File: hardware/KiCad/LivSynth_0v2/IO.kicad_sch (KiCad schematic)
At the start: 95 parts, among them J1 PJ398SM, J13 Jumper, J14 Jumper, J2 PJ398SM, J20 IDC, J3 PJ398SM, J4 IDC, Q6 2N3904, Q7 2N3904, SW6 SW_Push, U10 PCA9685PW, U11 PCA9685PW, U13 74HC165, U14 74HC165, U3 LM386

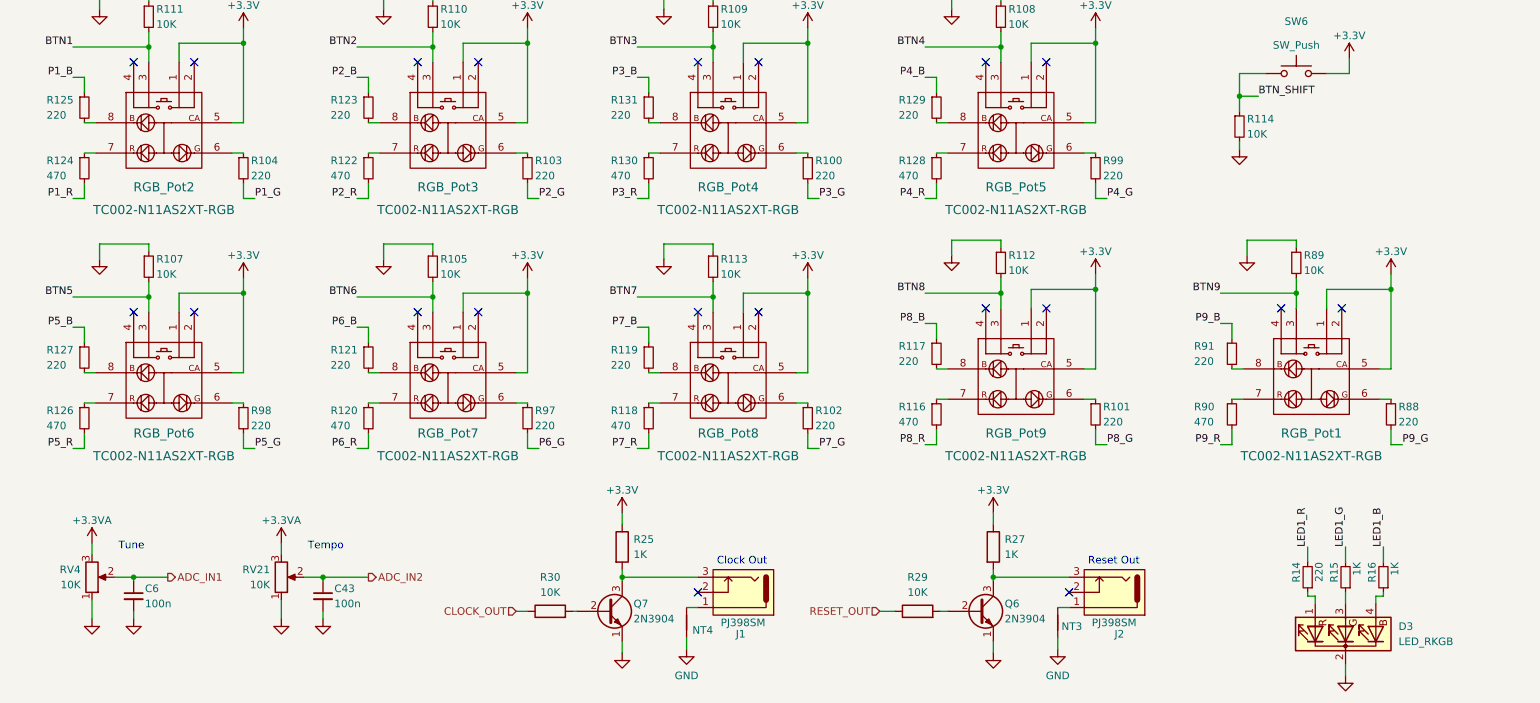
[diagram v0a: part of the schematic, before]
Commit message: Create new 0v3 folder
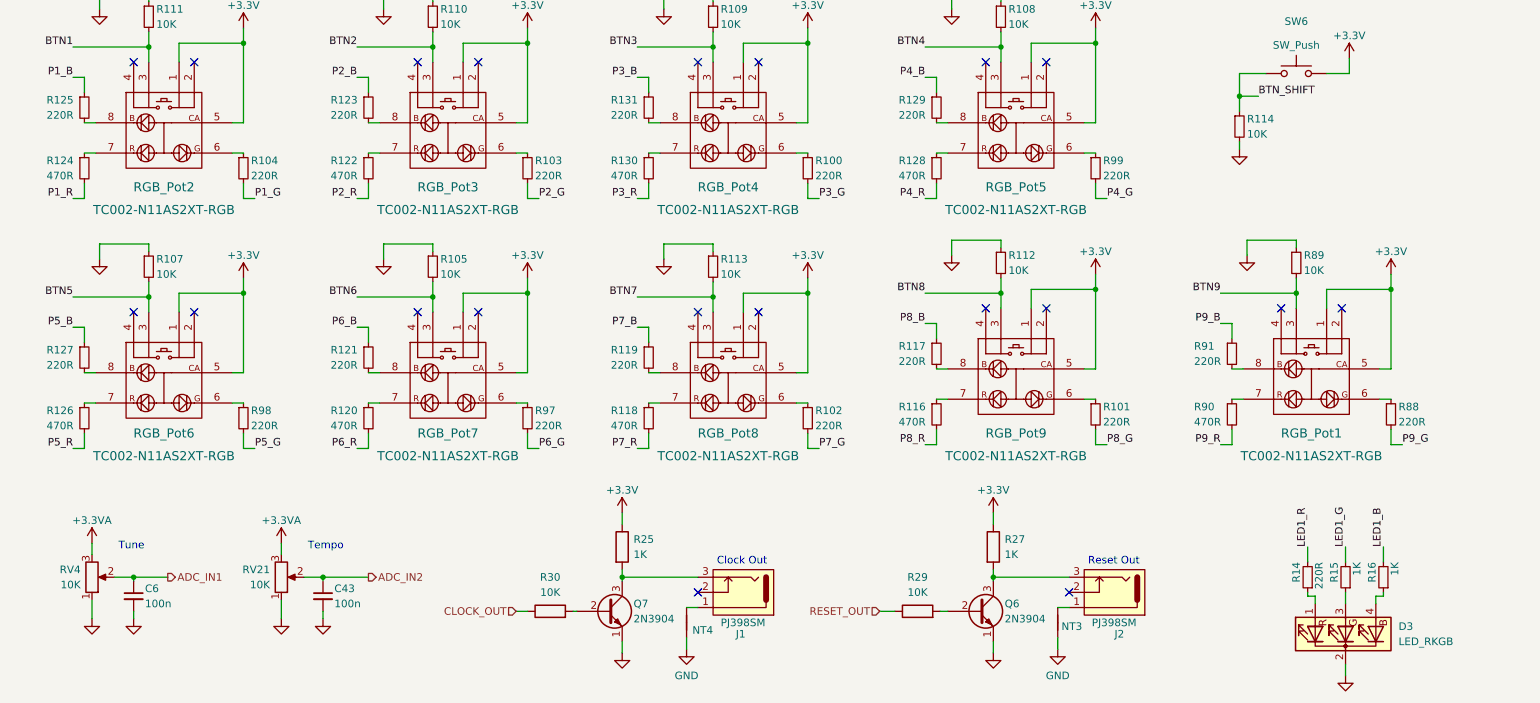
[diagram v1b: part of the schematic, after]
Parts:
- R100, R101, R102, R103, R104, R117, R119, R121, R123, R125, R127, R129, R131, R14, R88, R91, R97, R98, R99: value 220 -> 220R
- R116, R118, R120, R122, R124, R126, R128, R130, R90: value 470 -> 470R
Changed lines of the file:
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@@
       (effects (font (size 1.27 1.27)) (justify left))
     )
-    (property "Value" "220" (id 1) (at 194.31 158.115 0)
+    (property "Value" "220R" (id 1) (at 194.31 158.115 0)
       (effects (font (size 1.27 1.27)) (justify left))
     )
@@
       (effects (font (size 1.27 1.27)) (justify left))
     )
-    (property "Value" "220" (id 1) (at 209.55 147.955 0)
+    (property "Value" "220R" (id 1) (at 209.55 147.955 0)
       (effects (font (size 1.27 1.27)) (justify left))
     )
@@
       (effects (font (size 1.27 1.27)) (justify left))
     )
-    (property "Value" "220" (id 1) (at 111.76 106.68 0)
+    (property "Value" "220R" (id 1) (at 111.76 106.68 0)
       (effects (font (size 1.27 1.27)) (justify left))
     )
@@
       (effects (font (size 1.27 1.27)) (justify left))
     )
-    (property "Value" "220" (id 1) (at 230.505 181.61 90)
+    (property "Value" "220R" (id 1) (at 230.505 181.61 90)
       (effects (font (size 1.27 1.27)) (justify left))
     )
@@
       (effects (font (size 1.27 1.27)) (justify left))
     )
-    (property "Value" "220" (id 1) (at 51.435 116.84 0)
+    (property "Value" "220R" (id 1) (at 51.435 116.84 0)
       (effects (font (size 1.27 1.27)) (justify left))
     )
@@
       (effects (font (size 1.27 1.27)) (justify left))
     )
-    (property "Value" "470" (id 1) (at 111.76 158.75 0)
+    (property "Value" "470R" (id 1) (at 111.76 158.75 0)
       (effects (font (size 1.27 1.27)) (justify left))
     )
@@
       (effects (font (size 1.27 1.27)) (justify left))
     )
-    (property "Value" "220" (id 1) (at 160.02 147.955 0)
+    (property "Value" "220R" (id 1) (at 160.02 147.955 0)
       (effects (font (size 1.27 1.27)) (justify left))
     )
@@
       (effects (font (size 1.27 1.27)) (justify left))
     )
-    (property "Value" "220" (id 1) (at 146.05 158.75 0)
+    (property "Value" "220R" (id 1) (at 146.05 158.75 0)
       (effects (font (size 1.27 1.27)) (justify left))
     )
@@
       (effects (font (size 1.27 1.27)) (justify left))
     )
-    (property "Value" "220" (id 1) (at 111.76 148.59 0)
+    (property "Value" "220R" (id 1) (at 111.76 148.59 0)
       (effects (font (size 1.27 1.27)) (justify left))
     )
@@
       (effects (font (size 1.27 1.27)) (justify left))
     )
-    (property "Value" "220" (id 1) (at 99.06 158.75 0)
+    (property "Value" "220R" (id 1) (at 99.06 158.75 0)
       (effects (font (size 1.27 1.27)) (justify left))
     )
@@
       (effects (font (size 1.27 1.27)) (justify left))
     )
-    (property "Value" "470" (id 1) (at 209.55 158.115 0)
+    (property "Value" "470R" (id 1) (at 209.55 158.115 0)
       (effects (font (size 1.27 1.27)) (justify left))
     )
@@
       (effects (font (size 1.27 1.27)) (justify left))
     )
-    (property "Value" "220" (id 1) (at 64.77 148.59 0)
+    (property "Value" "220R" (id 1) (at 64.77 148.59 0)
       (effects (font (size 1.27 1.27)) (justify left))
     )
@@
       (effects (font (size 1.27 1.27)) (justify left))
     )
-    (property "Value" "220" (id 1) (at 194.31 116.84 0)
+    (property "Value" "220R" (id 1) (at 194.31 116.84 0)
       (effects (font (size 1.27 1.27)) (justify left))
     )
@@
       (effects (font (size 1.27 1.27)) (justify left))
     )
-    (property "Value" "220" (id 1) (at 17.145 106.68 0)
+    (property "Value" "220R" (id 1) (at 17.145 106.68 0)
       (effects (font (size 1.27 1.27)) (justify left))
     )
@@
       (effects (font (size 1.27 1.27)) (justify left))
     )
-    (property "Value" "220" (id 1) (at 51.435 158.75 0)
+    (property "Value" "220R" (id 1) (at 51.435 158.75 0)
       (effects (font (size 1.27 1.27)) (justify left))
     )
@@
       (effects (font (size 1.27 1.27)) (justify left))
     )
-    (property "Value" "470" (id 1) (at 111.76 116.84 0)
+    (property "Value" "470R" (id 1) (at 111.76 116.84 0)
       (effects (font (size 1.27 1.27)) (justify left))
     )
@@
       (effects (font (size 1.27 1.27)) (justify left))
     )
-    (property "Value" "470" (id 1) (at 17.145 116.84 0)
+    (property "Value" "470R" (id 1) (at 17.145 116.84 0)
       (effects (font (size 1.27 1.27)) (justify left))
     )
@@
       (effects (font (size 1.27 1.27)) (justify left))
     )
-    (property "Value" "220" (id 1) (at 243.84 158.115 0)
+    (property "Value" "220R" (id 1) (at 243.84 158.115 0)
       (effects (font (size 1.27 1.27)) (justify left))
     )
@@
       (effects (font (size 1.27 1.27)) (justify left))
     )
-    (property "Value" "220" (id 1) (at 99.06 116.84 0)
+    (property "Value" "220R" (id 1) (at 99.06 116.84 0)
       (effects (font (size 1.27 1.27)) (justify left))
     )
@@
       (effects (font (size 1.27 1.27)) (justify left))
     )
-    (property "Value" "470" (id 1) (at 64.77 116.84 0)
+    (property "Value" "470R" (id 1) (at 64.77 116.84 0)
       (effects (font (size 1.27 1.27)) (justify left))
     )
@@
       (effects (font (size 1.27 1.27)) (justify left))
     )
-    (property "Value" "470" (id 1) (at 64.77 158.75 0)
+    (property "Value" "470R" (id 1) (at 64.77 158.75 0)
       (effects (font (size 1.27 1.27)) (justify left))
     )
@@
       (effects (font (size 1.27 1.27)) (justify left))
     )
-    (property "Value" "220" (id 1) (at 160.02 106.68 0)
+    (property "Value" "220R" (id 1) (at 160.02 106.68 0)
       (effects (font (size 1.27 1.27)) (justify left))
     )
@@
       (effects (font (size 1.27 1.27)) (justify left))
     )
-    (property "Value" "220" (id 1) (at 146.05 116.84 0)
+    (property "Value" "220R" (id 1) (at 146.05 116.84 0)
       (effects (font (size 1.27 1.27)) (justify left))
     )
@@
       (effects (font (size 1.27 1.27)) (justify left))
     )
-    (property "Value" "470" (id 1) (at 160.02 116.84 0)
+    (property "Value" "470R" (id 1) (at 160.02 116.84 0)
       (effects (font (size 1.27 1.27)) (justify left))
     )
@@
       (effects (font (size 1.27 1.27)) (justify left))
     )
-    (property "Value" "220" (id 1) (at 64.77 106.68 0)
+    (property "Value" "220R" (id 1) (at 64.77 106.68 0)
       (effects (font (size 1.27 1.27)) (justify left))
     )
@@
       (effects (font (size 1.27 1.27)) (justify left))
     )
-    (property "Value" "470" (id 1) (at 160.02 158.115 0)
+    (property "Value" "470R" (id 1) (at 160.02 158.115 0)
       (effects (font (size 1.27 1.27)) (justify left))
     )
@@
       (effects (font (size 1.27 1.27)) (justify left))
     )
-    (property "Value" "220" (id 1) (at 17.145 148.59 0)
+    (property "Value" "220R" (id 1) (at 17.145 148.59 0)
       (effects (font (size 1.27 1.27)) (justify left))
     )
@@
       (effects (font (size 1.27 1.27)) (justify left))
     )
-    (property "Value" "470" (id 1) (at 17.145 158.75 0)
-      (effects (font (size 1.27 1.27)) (justify left))
-    )
+    (property "Value" "470R" (id 1) (at 17.145 158.75 0)
+      (effects (font (size 1.27 1.27)) (justify left))
+    )
